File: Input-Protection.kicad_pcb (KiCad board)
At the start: 2 copper layers, 80 x 50 mm, 77 parts, among them J101 KLDX-0202-B, J102 EBWA-02-B, J103 EBWA-02-B, J104 KLDX-0202-B, Q201 MCU18P10Y-TP, Q601 BC846, Q602 MCU18P10Y-TP, U401 LM4040N-5.0, U501 LM393, U502 LM393, U503 INA169NA/3K

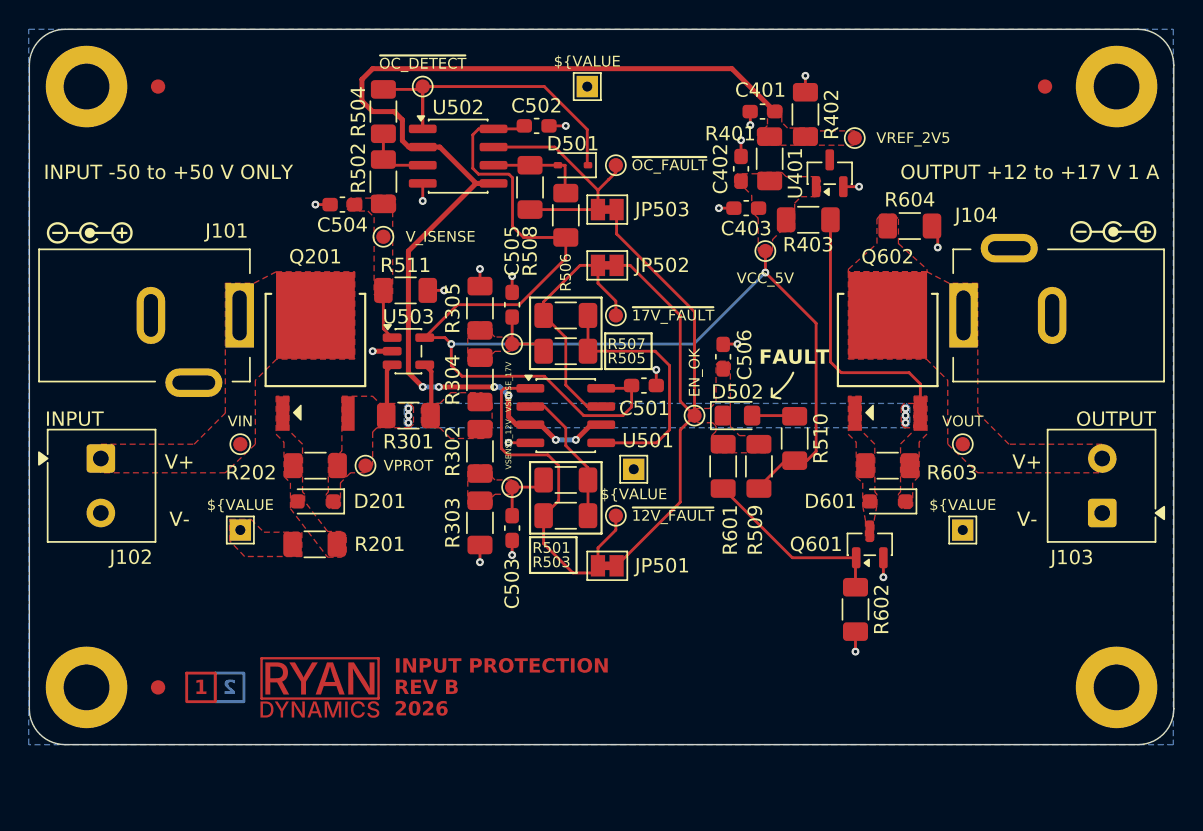
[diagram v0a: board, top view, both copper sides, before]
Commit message: feat: pcb mvp
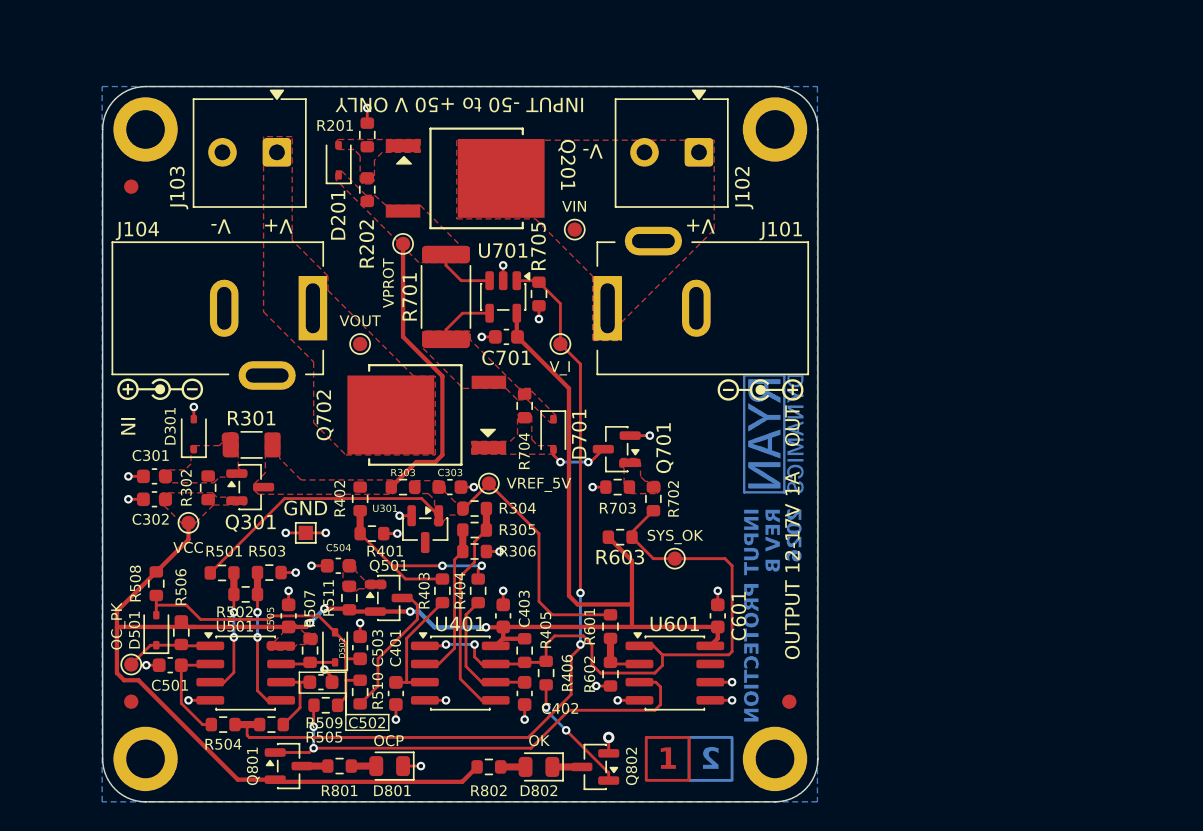
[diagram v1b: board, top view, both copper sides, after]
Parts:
- removed C506: 1u, Capacitor_SMD:C_0603_1608Metric_Pad1.08x0.95mm_HandSolder
- removed D601: D3Z10BF-7, Diode_SMD:D_SOD-323_HandSoldering
- removed JP501, JP502, JP503: SolderJumper_2_Bridged, Jumper:SolderJumper-2_P1.3mm_Bridged_Pad1.0x1.5mm
- removed Q601: BC846, Package_TO_SOT_SMD:SOT-23
- removed Q602: MCU18P10Y-TP, MCU18P10Y-TP:DPAK_MCC
- removed R604: 1M, Resistor_SMD:R_1206_3216Metric_Pad1.30x1.75mm_HandSolder
- removed TP103: VOUT, RD-Testpoints:TestPoint_Pad_D1.0mm
- removed TP104, TP507: GND, RD-Testpoints:TestPoint_THTPad_1.5x1.5mm_Drill0.7mm
- removed TP303: VSENSE_17V, RD-Testpoints:TestPoint_Pad_D1.0mm
- removed TP401: VREF_2V5, RD-Testpoints:TestPoint_Pad_D1.0mm
- removed TP402: VCC_5V, RD-Testpoints:TestPoint_Pad_D1.0mm
- removed TP502: ~{OC_DETECT}, RD-Testpoints:TestPoint_Pad_D1.0mm
- removed TP503: ~{17V_FAULT}, RD-Testpoints:TestPoint_Pad_D1.0mm
- removed TP504: ~{OC_FAULT}, RD-Testpoints:TestPoint_Pad_D1.0mm
- removed TP505: V_ISENSE, RD-Testpoints:TestPoint_Pad_D1.0mm
- removed TP506: EN_OK, RD-Testpoints:TestPoint_Pad_D1.0mm
- removed U502: LM393, Package_SO:SOIC-8_3.9x4.9mm_P1.27mm
- removed U503: INA169NA/3K, Package_TO_SOT_SMD:SOT-23-5
- added C301: 100n, Capacitor_SMD:C_0603_1608Metric, F.Cu at (126.3, 82.9)
- added C302: 1u, Capacitor_SMD:C_0603_1608Metric, F.Cu at (126.3, 84.5)
- added C303: 10n, Capacitor_SMD:C_0603_1608Metric, F.Cu at (147.0, 83.7)
- added C601: 100n, Capacitor_SMD:C_0603_1608Metric, F.Cu at (165.7, 92.7)
- added C701: 100n, Capacitor_SMD:C_0603_1608Metric, F.Cu at (150.9, 73.2)
- added D301: MM3Z5V6, Diode_SMD:D_SOD-323, F.Cu at (129.1, 80.0)
- added D701: D3Z10BF-7, Diode_SMD:D_SOD-323, F.Cu at (154.2, 80.0)
- added D801: LED, LED_SMD:LED_0805_2012Metric, F.Cu at (142.8, 103.2)
- added D802: LED, LED_SMD:LED_0805_2012Metric, F.Cu at (153.2, 103.2)
- added Q301: BC846, Package_TO_SOT_SMD:SOT-23, F.Cu at (133.0, 83.7)
- added Q501: BC856, Package_TO_SOT_SMD:SOT-23, F.Cu at (142.7, 91.4)
- added Q701: BC846, Package_TO_SOT_SMD:SOT-23, F.Cu at (158.6, 81.0)
- added Q702: MCU18P10Y-TP, MCU18P10Y-TP:DPAK_MCC, F.Cu at (144.5, 78.6)
- added Q801: BC856, Package_TO_SOT_SMD:SOT-23, F.Cu at (135.7, 103.2)
- added Q802: BC846, Package_TO_SOT_SMD:SOT-23, F.Cu at (157.1, 103.2)
- added R306: 121k, Resistor_SMD:R_0603_1608Metric, F.Cu at (148.7, 88.2)
- added R404: 1k, Resistor_SMD:R_0603_1608Metric, F.Cu at (148.9, 90.9)
- added R405: 10k, Resistor_SMD:R_0603_1608Metric, F.Cu at (152.2, 95.1)
- added R406: 100k, Resistor_SMD:R_0603_1608Metric, F.Cu at (153.7, 96.7)
- added R701: 20m, Resistor_SMD:R_2512_6332Metric, F.Cu at (146.7, 70.4)
- added R702: 10k, Resistor_SMD:R_0603_1608Metric, F.Cu at (161.2, 84.5)
- added R703: 100k, Resistor_SMD:R_0603_1608Metric, F.Cu at (158.7, 83.7)
- added R704: 100k, Resistor_SMD:R_0603_1608Metric, F.Cu at (152.2, 78.0)
- added R705: 15k, Resistor_SMD:R_0603_1608Metric, F.Cu at (153.2, 70.2)
- added R801: 2.49k, Resistor_SMD:R_0603_1608Metric, F.Cu at (139.3, 103.1)
- added R802: 2.49k, Resistor_SMD:R_0603_1608Metric, F.Cu at (149.7, 103.2)
- added TP701: SYS_OK, RD-Testpoints:TestPoint_Pad_D1.0mm, F.Cu at (162.7, 88.7)
- added TP702: V_I, RD-Testpoints:TestPoint_Pad_D1.0mm, F.Cu at (154.7, 73.7)
- added TP901: GND, RD-Testpoints:TestPoint_Pad_1.0x1.0mm, F.Cu at (136.9, 86.8)
- added U301: LM4040N-5.0, Package_TO_SOT_SMD:SOT-23, F.Cu at (145.2, 86.6)
- added U601: LM393, Package_SO:SOIC-8_3.9x4.9mm_P1.27mm, F.Cu at (162.7, 96.7)
- added U701: INA169NA/3K, Package_TO_SOT_SMD:SOT-23-5, F.Cu at (150.7, 70.4)
- C401, C403: footprint Capacitor_SMD:C_0603_1608Metric_Pad1.08x0.95mm_HandSolder -> Capacitor_SMD:C_0603_1608Metric
- C402: value 1u -> 10n; footprint Capacitor_SMD:C_0603_1608Metric_Pad1.08x0.95mm_HandSolder -> Capacitor_SMD:C_0603_1608Metric
- C501: value 100n -> 10n; footprint Capacitor_SMD:C_0603_1608Metric_Pad1.08x0.95mm_HandSolder -> Capacitor_SMD:C_0603_1608Metric
- C502: value 100n -> 1u; footprint Capacitor_SMD:C_0603_1608Metric_Pad1.08x0.95mm_HandSolder -> Capacitor_SMD:C_0603_1608Metric
- C503: value 10n -> 4.7u; footprint Capacitor_SMD:C_0603_1608Metric_Pad1.08x0.95mm_HandSolder -> Capacitor_SMD:C_0603_1608Metric
- C504: value 10n -> 1u; footprint Capacitor_SMD:C_0603_1608Metric_Pad1.08x0.95mm_HandSolder -> Capacitor_SMD:C_0603_1608Metric
- C505: value 10n -> 100n; footprint Capacitor_SMD:C_0603_1608Metric_Pad1.08x0.95mm_HandSolder -> Capacitor_SMD:C_0603_1608Metric
- D201: footprint Diode_SMD:D_SOD-323_HandSoldering -> Diode_SMD:D_SOD-323
- D502: value LED -> 1N4148WS; footprint LED_SMD:LED_0805_2012Metric_Pad1.15x1.40mm_HandSolder -> Diode_SMD:D_SOD-323
- H901, H902, H903, H904: value MOUNT_M3 -> MOUNT_M2.5; footprint MountingHole:MountingHole_3.2mm_M3_ISO7380_Pad -> MountingHole:MountingHole_2.7mm_M2.5_ISO7380_Pad
- ID901: footprint RD-Symbols-Silkscreen:STACKUP_ID_2L_SML -> RD-Symbols-Silkscreen:STACKUP_ID_2L
- R201, R202: footprint Resistor_SMD:R_1206_3216Metric_Pad1.30x1.75mm_HandSolder -> Resistor_SMD:R_0603_1608Metric
- R301: value 100m -> 12.1k; footprint Resistor_SMD:R_1206_3216Metric_Pad1.30x1.75mm_HandSolder -> Resistor_SMD:R_1206_3216Metric
- R302: value 39.2k -> 100k; footprint Resistor_SMD:R_1206_3216Metric_Pad1.30x1.75mm_HandSolder -> Resistor_SMD:R_0603_1608Metric
- R303: value 10k -> 33.2k; footprint Resistor_SMD:R_1206_3216Metric_Pad1.30x1.75mm_HandSolder -> Resistor_SMD:R_0603_1608Metric
- R304: value 56.2k -> 332k; footprint Resistor_SMD:R_1206_3216Metric_Pad1.30x1.75mm_HandSolder -> Resistor_SMD:R_0603_1608Metric
- R305: value 10k -> 49.9k; footprint Resistor_SMD:R_1206_3216Metric_Pad1.30x1.75mm_HandSolder -> Resistor_SMD:R_0603_1608Metric
- R401: value 100k -> 22.1k; footprint Resistor_SMD:R_1206_3216Metric_Pad1.30x1.75mm_HandSolder -> Resistor_SMD:R_0603_1608Metric
- R402: value 100k -> 200k; footprint Resistor_SMD:R_1206_3216Metric_Pad1.30x1.75mm_HandSolder -> Resistor_SMD:R_0603_1608Metric
- R403, R510: value 3.32k -> 1k; footprint Resistor_SMD:R_1206_3216Metric_Pad1.30x1.75mm_HandSolder -> Resistor_SMD:R_0603_1608Metric
- R501: value 1k -> 357k; footprint Resistor_SMD:R_1206_3216Metric_Pad1.30x1.75mm_HandSolder -> Resistor_SMD:R_0603_1608Metric
- R502: value 1k -> 121k; footprint Resistor_SMD:R_1206_3216Metric_Pad1.30x1.75mm_HandSolder -> Resistor_SMD:R_0603_1608Metric
- R503: value 1M -> 30.1k; footprint Resistor_SMD:R_1206_3216Metric_Pad1.30x1.75mm_HandSolder -> Resistor_SMD:R_0603_1608Metric
- R504: value 1M -> 1k; footprint Resistor_SMD:R_1206_3216Metric_Pad1.30x1.75mm_HandSolder -> Resistor_SMD:R_0603_1608Metric
- R505: value 1k -> 49.9k; footprint Resistor_SMD:R_1206_3216Metric_Pad1.30x1.75mm_HandSolder -> Resistor_SMD:R_0603_1608Metric
- R506, R603: value 100k -> 10k; footprint Resistor_SMD:R_1206_3216Metric_Pad1.30x1.75mm_HandSolder -> Resistor_SMD:R_0603_1608Metric
- R507: value 1M -> 10k; footprint Resistor_SMD:R_1206_3216Metric_Pad1.30x1.75mm_HandSolder -> Resistor_SMD:R_0603_1608Metric
- R508: value 10k -> 432k; footprint Resistor_SMD:R_1206_3216Metric_Pad1.30x1.75mm_HandSolder -> Resistor_SMD:R_0603_1608Metric
- R509: value 10k -> 100k; footprint Resistor_SMD:R_1206_3216Metric_Pad1.30x1.75mm_HandSolder -> Resistor_SMD:R_0603_1608Metric
- R511: value 22.1k -> 100k; footprint Resistor_SMD:R_1206_3216Metric_Pad1.30x1.75mm_HandSolder -> Resistor_SMD:R_0603_1608Metric
- R601: value 10k -> 18.2k; footprint Resistor_SMD:R_1206_3216Metric_Pad1.30x1.75mm_HandSolder -> Resistor_SMD:R_0603_1608Metric
- R602: value 100k -> 33.2k; footprint Resistor_SMD:R_1206_3216Metric_Pad1.30x1.75mm_HandSolder -> Resistor_SMD:R_0603_1608Metric
- TP101: value GND -> VIN; footprint RD-Testpoints:TestPoint_THTPad_1.5x1.5mm_Drill0.7mm -> RD-Testpoints:TestPoint_Pad_D1.0mm
- TP102: value VIN -> VOUT
- TP301: value GND -> VCC; footprint RD-Testpoints:TestPoint_THTPad_1.5x1.5mm_Drill0.7mm -> RD-Testpoints:TestPoint_Pad_D1.0mm
- TP302: value VSENSE_12V -> VREF_5V
- TP501: value ~{12V_FAULT} -> OC_PK
- U401: value LM4040N-5.0 -> LM393; footprint Package_TO_SOT_SMD:SOT-23 -> Package_SO:SOIC-8_3.9x4.9mm_P1.27mm
- moved H904 68.1 mm to (125.7, 102.7)
- moved J103 63.0 mm to (134.9, 60.2), turned to 180 degrees
- moved H902 61.9 mm to (169.7, 58.6)
- moved H903 52.7 mm to (169.7, 102.7)
- moved C401 48.1 mm to (143.2, 98.1), turned to 90 degrees
- moved J102 47.0 mm to (164.4, 60.2), turned to 180 degrees
- moved FID903 46.6 mm to (170.7, 98.7)
- moved J104 45.5 mm to (137.4, 71.2), turned to 0 degrees
- moved R504 44.3 mm to (131.1, 100.2), turned to 0 degrees
- moved D501 43.6 mm to (126.4, 93.7), turned to 90 degrees
- moved U401 43.4 mm to (147.7, 96.7), turned to 0 degrees
- moved C502 41.7 mm to (138.0, 97.3)
- moved R402 41.1 mm to (140.7, 84.5), turned to 90 degrees
- moved C402 39.7 mm to (152.2, 98.1)
- moved R506 39.7 mm to (128.2, 93.8), turned to 90 degrees
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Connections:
- C401 pad 1: VREF_2V5 -> GND
- C401 pad 2: GND -> /SCHEMATIC/V_SENSE_UV
- C402 pad 1: VCC_5V -> GND
- C402 pad 2: GND -> /SCHEMATIC/V_SENSE_OV
- C403 pad 1: VCC_5V -> VCC
- C501 pad 1: VCC_5V -> /SCHEMATIC/I_SENSE_PEAK
- C502 pad 1: VCC_5V -> /SCHEMATIC/I_SENSE_1A
- C503 pad 1: GND -> /SCHEMATIC/OC_LOCKOUT
- C503 pad 2: /ARCHITECTURE/3. SENSING/VSENSE_12V -> GND
- C504 pad 1: /ARCHITECTURE/5. COMPARATOR/V_ISENSE -> /SCHEMATIC/B_PRCHRG
- C505 pad 1: /ARCHITECTURE/3. SENSING/VSENSE_17V -> VCC
- D201 pad 1: /ARCHITECTURE/2. POLARITY PROTECTION/VPROT -> VPROT
- D201 pad 2: Net-(D201-A) -> /SCHEMATIC/GATE_RPP
- D501 pad 1: /ARCHITECTURE/5. COMPARATOR/~{OC_DETECT} -> /SCHEMATIC/OC_PEAK_FAULT
- D501 pad 2: /ARCHITECTURE/5. COMPARATOR/LATCH_IN -> /SCHEMATIC/OC_LOCKOUT
- D502 pad 1: /ARCHITECTURE/5. COMPARATOR/EN_OK -> /SCHEMATIC/OC_1A_FAULT
- D502 pad 2: Net-(D502-A) -> /SCHEMATIC/OC_LOCKOUT
- J101 pad 1: /ARCHITECTURE/1. INTERCONNECTS/VIN -> VIN
- J102 pad 1: /ARCHITECTURE/1. INTERCONNECTS/VIN -> VIN
- J103 pad 1: GND -> VOUT
- J103 pad 2: /ARCHITECTURE/1. INTERCONNECTS/VOUT -> GND
- J104 pad 1: /ARCHITECTURE/1. INTERCONNECTS/VOUT -> VOUT
- Q201 pad 1: Net-(D201-A) -> /SCHEMATIC/GATE_RPP
- Q201 pad 2: /ARCHITECTURE/1. INTERCONNECTS/VIN -> VIN
- Q201 pad 3: /ARCHITECTURE/2. POLARITY PROTECTION/VPROT -> VPROT
- R201 pad 1: GND -> /SCHEMATIC/GATE_RPP
- R201 pad 2: Net-(D201-A) -> GND
- R202 pad 1: Net-(D201-A) -> /SCHEMATIC/GATE_RPP
- R202 pad 2: /ARCHITECTURE/2. POLARITY PROTECTION/VPROT -> VPROT
- R301 pad 1: /ARCHITECTURE/3. SENSING/ISENSE_N -> /SCHEMATIC/VZ
- R301 pad 2: /ARCHITECTURE/2. POLARITY PROTECTION/VPROT -> VPROT
- R302 pad 1: /ARCHITECTURE/3. SENSING/VSENSE_12V -> /SCHEMATIC/VZ
- R302 pad 2: /ARCHITECTURE/3. SENSING/ISENSE_N -> VCC
- R303 pad 1: GND -> VREF_5V
- R303 pad 2: /ARCHITECTURE/3. SENSING/VSENSE_12V -> VPROT
- R304 pad 1: /ARCHITECTURE/3. SENSING/VSENSE_17V -> VREF_5V
- R304 pad 2: /ARCHITECTURE/3. SENSING/ISENSE_N -> OV_REF
- R305 pad 1: GND -> UV_REF
- R305 pad 2: /ARCHITECTURE/3. SENSING/VSENSE_17V -> OV_REF
- R401 pad 1: VREF_2V5 -> GND
- R401 pad 2: VCC_5V -> /SCHEMATIC/V_SENSE
- R402 pad 1: GND -> /SCHEMATIC/V_SENSE
- R402 pad 2: VREF_2V5 -> VPROT
- R403 pad 1: VCC_5V -> /SCHEMATIC/V_SENSE_UV
- R403 pad 2: /ARCHITECTURE/2. POLARITY PROTECTION/VPROT -> /SCHEMATIC/V_SENSE
- R501 pad 1: Net-(U501A--) -> /SCHEMATIC/OC_PEAK_REF
- R501 pad 2: /ARCHITECTURE/3. SENSING/VSENSE_12V -> VREF_5V
- R502 pad 1: /ARCHITECTURE/5. COMPARATOR/V_ISENSE -> /SCHEMATIC/OC_1A_REF
- R502 pad 2: Net-(U502A-+) -> /SCHEMATIC/OC_PEAK_REF
- R503 pad 1: Net-(U501A--) -> GND
- R503 pad 2: /ARCHITECTURE/5. COMPARATOR/~{12V_FAULT} -> /SCHEMATIC/OC_1A_REF
- R504 pad 1: Net-(U502A-+) -> /SCHEMATIC/I_SENSE_PEAK
- R504 pad 2: /ARCHITECTURE/5. COMPARATOR/~{OC_DETECT} -> V_I
- R505 pad 1: /ARCHITECTURE/3. SENSING/VSENSE_17V -> /SCHEMATIC/I_SENSE_1A
- R505 pad 2: Net-(U501B-+) -> V_I
- R506 pad 1: /ARCHITECTURE/5. COMPARATOR/LATCH_IN -> /SCHEMATIC/OC_PEAK_FAULT
- R506 pad 2: VCC_5V -> VCC
- R507 pad 1: Net-(U501B-+) -> /SCHEMATIC/OC_1A_FAULT
- R507 pad 2: /ARCHITECTURE/5. COMPARATOR/~{17V_FAULT} -> VCC
- R508 pad 1: /ARCHITECTURE/5. COMPARATOR/LATCH_IN -> /SCHEMATIC/OC_LOCKOUT
- R508 pad 2: /ARCHITECTURE/5. COMPARATOR/~{OC_FAULT} -> VCC
- R509 pad 1: /ARCHITECTURE/5. COMPARATOR/EN_OK -> OC_FAULT
- R509 pad 2: VCC_5V -> /SCHEMATIC/OC_LOCKOUT
- R510 pad 1: Net-(D502-A) -> /SCHEMATIC/CAP_PRCHRG
- R510 pad 2: VCC_5V -> /SCHEMATIC/OC_LOCKOUT
- R511 pad 1: GND -> VCC
- R511 pad 2: /ARCHITECTURE/5. COMPARATOR/V_ISENSE -> /SCHEMATIC/B_PRCHRG
- R601 pad 1: Net-(Q601-B) -> /SCHEMATIC/OC_LOCKOUT_REF
- R601 pad 2: /ARCHITECTURE/5. COMPARATOR/EN_OK -> VREF_5V
- R602 pad 1: Net-(Q601-B) -> GND
- R602 pad 2: GND -> /SCHEMATIC/OC_LOCKOUT_REF
- R603 pad 1: Net-(D601-A) -> SYS_OK
- R603 pad 2: /ARCHITECTURE/2. POLARITY PROTECTION/VPROT -> VCC
- TP101 pad 1: GND -> VIN
- TP102 pad 1: /ARCHITECTURE/1. INTERCONNECTS/VIN -> VOUT
- TP201 pad 1: /ARCHITECTURE/2. POLARITY PROTECTION/VPROT -> VPROT
- TP301 pad 1: GND -> VCC
- TP302 pad 1: /ARCHITECTURE/3. SENSING/VSENSE_12V -> VREF_5V
- TP501 pad 1: /ARCHITECTURE/5. COMPARATOR/~{12V_FAULT} -> /SCHEMATIC/OC_PEAK_FAULT
- U401 pad 1: VCC_5V -> SYS_OK
- U401 pad 2: GND -> UV_REF
- U401 pad 3: unconnected-(U401-NC-Pad3) -> /SCHEMATIC/V_SENSE_UV
- U501 pad 1: /ARCHITECTURE/5. COMPARATOR/~{12V_FAULT} -> /SCHEMATIC/OC_PEAK_FAULT
- U501 pad 2: Net-(U501A--) -> /SCHEMATIC/I_SENSE_PEAK
- U501 pad 3: VREF_2V5 -> /SCHEMATIC/OC_PEAK_REF
- U501 pad 5: Net-(U501B-+) -> /SCHEMATIC/OC_1A_REF
- U501 pad 6: VREF_2V5 -> /SCHEMATIC/I_SENSE_1A
- U501 pad 7: /ARCHITECTURE/5. COMPARATOR/~{17V_FAULT} -> /SCHEMATIC/OC_1A_FAULT
- U501 pad 8: VCC_5V -> VCC
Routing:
- net VCC: track 0.00 -> 123.8 mm, vias 0 -> 4
- net VCC_5V: track 96.6 -> 0.00 mm, vias 2 -> 0
- net VREF_2V5: track 76.3 -> 0.00 mm, vias 6 -> 0
- net V_I: track 0.00 -> 58.3 mm, vias 0 -> 2
- net SYS_OK: track 0.00 -> 45.2 mm, vias 0 -> 2
- net /ARCHITECTURE/5. COMPARATOR/EN_OK: track 42.8 -> 0.00 mm
- net VREF_5V: track 0.00 -> 36.3 mm
- net OC_FAULT: track 0.00 -> 34.2 mm, vias 0 -> 2
- net /ARCHITECTURE/5. COMPARATOR/~{12V_FAULT}: track 25.7 -> 0.00 mm
- net VPROT: track 0.00 -> 24.6 mm
- net /ARCHITECTURE/5. COMPARATOR/~{OC_DETECT}: track 23.8 -> 0.00 mm
- net /ARCHITECTURE/2. POLARITY PROTECTION/VPROT: track 22.6 -> 0.00 mm, vias 6 -> 0
- net /SCHEMATIC/OC_LOCKOUT: track 0.00 -> 22.5 mm
- net /ARCHITECTURE/5. COMPARATOR/~{17V_FAULT}: track 18.4 -> 0.00 mm
- net Net-(U501B-+): track 18.3 -> 0.00 mm
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- added copper zone on F.Cu, net /SCHEMATIC/B_PRCHRG
- added copper zone on F.Cu, net /SCHEMATIC/GATE_P
- added copper zone on F.Cu, net /SCHEMATIC/GATE_RPP
- added copper zone on F.Cu, net /SCHEMATIC/VZ
- added copper zone on F.Cu, net Net-(Q701-B)
- added copper zone on F.Cu, net VCC
- added copper zone on F.Cu, net VIN
- added copper zone on F.Cu, net VOUT
- added copper zone on F.Cu, net VPROT
- added copper zone on F.Cu, net VREF_5V
- added copper zone on F.Cu, net VSUPPLY
- removed copper zone on F.Cu, net /ARCHITECTURE/1. INTERCONNECTS/VIN
- removed copper zone on F.Cu, net /ARCHITECTURE/1. INTERCONNECTS/VOUT
- removed copper zone on B.Cu, net /ARCHITECTURE/2. POLARITY PROTECTION/VPROT
- removed copper zone on F.Cu, net /ARCHITECTURE/2. POLARITY PROTECTION/VPROT
- removed copper zone on F.Cu, net /ARCHITECTURE/3. SENSING/ISENSE_N
- removed copper zone on F.Cu, net /ARCHITECTURE/3. SENSING/VSENSE_12V
- removed copper zone on F.Cu, net /ARCHITECTURE/3. SENSING/VSENSE_17V
- removed copper zone on F.Cu, net /ARCHITECTURE/5. COMPARATOR/EN_OK
- removed copper zone on F.Cu, net /ARCHITECTURE/5. COMPARATOR/V_ISENSE
- removed copper zone on F.Cu, net GND
- removed copper zone on F.Cu, net Net-(D201-A)
- removed copper zone on F.Cu, net Net-(D601-A)
- removed copper zone on F.Cu, net VCC_5V
- removed copper zone on F.Cu, net VREF_2V5
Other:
- board size 80 x 50 mm -> 50 x 50 mm
- board text added: "IN"
- board text added: "OCP"
- board text added: "OK"
- board text added: "OUT"
- board text added: "OUTPUT 12-17V 1A"
- board text removed: "FAULT"
- board text removed: "INPUT"
- board text removed: "OUTPUT"
- board text removed: "OUTPUT +12 to +17 V 1 A"
